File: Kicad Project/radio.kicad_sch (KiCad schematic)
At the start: 110 parts, among them CN20 DF40C-24DP-0.4V, J19 U.FL, J20 U.FL, Q1 MMBT3904-TP, SW3 SW_Push, SW4 SW_Push, U19 TXM27.12M0004322DBBDO00T, U20 CC1101RGPR, U21 0896BM15A0001001E, U22 LC29HBA, U23 EM4095HMSO16B+, U24 PE4259-63, U25 PE4259-63, U26 PE4259-63, U27 PE4259-63, U28 0433BM15A0001001E, U29 PN7160A1HN/C100E, U31 S2B-PH-K-S-GW, U32 S2B-PH-K-S-GW, U33 ESP32-S3-WROOM-1U-N16R2, U34 SiP32508DT, U35 SiP32508DT, U64 TCA9535PWR, U71 SKY13373-460LF, U72 SN74AXC1T45DCKR, Y3 26.0MHz

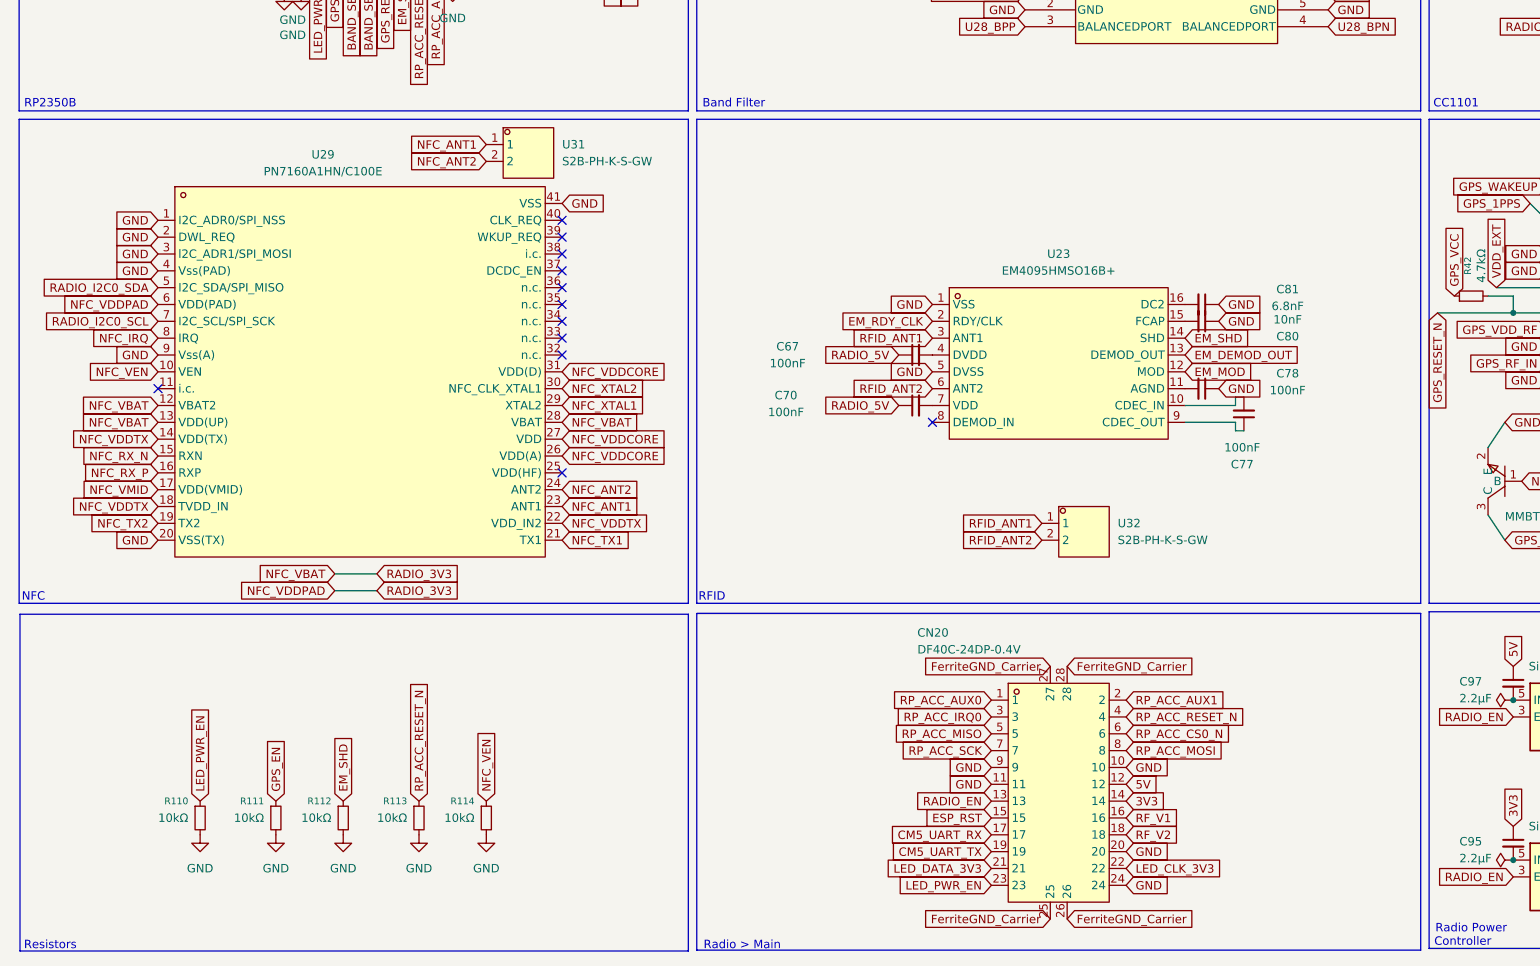
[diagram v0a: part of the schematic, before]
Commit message: added devlog and worked on NFC stack
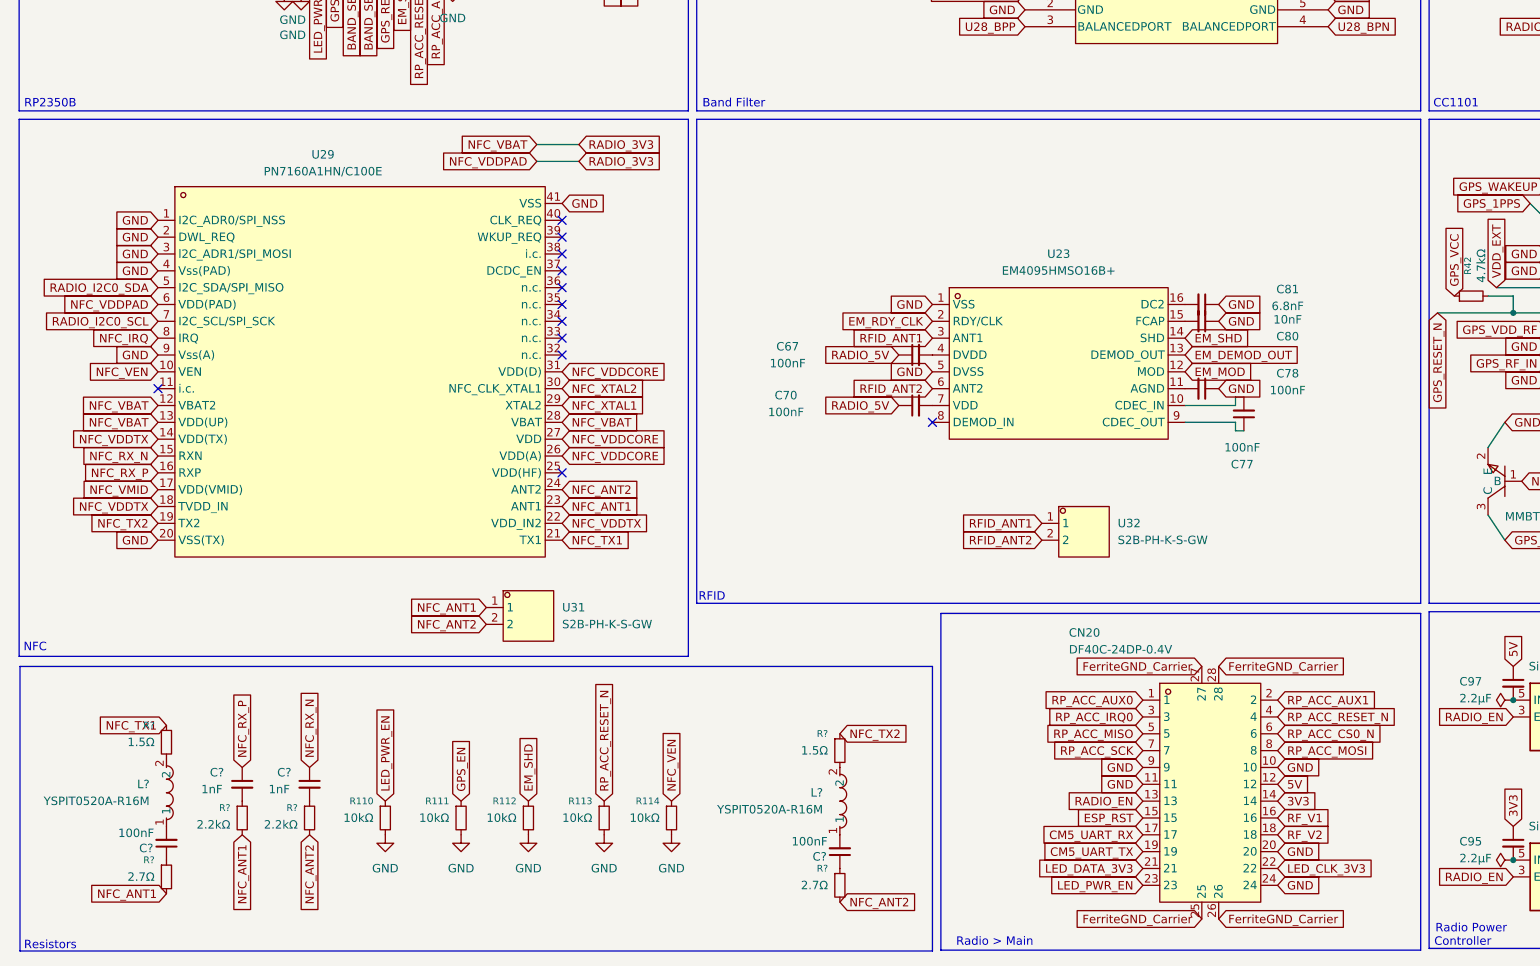
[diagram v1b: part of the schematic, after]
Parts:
- added C? (x2): 100nF, Capacitor_SMD:C_0402_1005Metric, symbol Device:C_Small
- added C? (x2): 1nF, Capacitor_SMD:C_0603_1608Metric, symbol Device:C_Small
- added L? (x2): YSPIT0520A-R16M, slate113:IND-SMD_L5.5-W5.3, symbol slate113:YSPIT0520A-R16M
- added R? (x2): 2.7Ω, Resistor_SMD:R_1206_3216Metric, symbol Device:R_Small
- added R? (x2): 2.2kΩ, Capacitor_SMD:C_0603_1608Metric, symbol Device:R_Small
- added R? (x2): 1.5Ω, Resistor_SMD:R_1206_3216Metric, symbol Device:R_Small
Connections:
- net NFC_ANT1: now also R?.2, R?.2
- net NFC_ANT2: now also R?.2, R?.2
- net NFC_RX_N: now also C?.1
- net NFC_RX_P: now also C?.1
- net NFC_TX1: now also R?.1
- net NFC_TX2: now also R?.1
- new net: C?.2, L?.1 (x2)
- new net: L?.2, R?.2 (x2)
- new net: C?.1, R?.1 (x2)
- new net: C?.2, R?.1 (x2)
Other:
- moved on the sheet: CN20, R110, R111, R112, R113, R114, U31
